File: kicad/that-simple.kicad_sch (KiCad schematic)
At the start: 20 parts

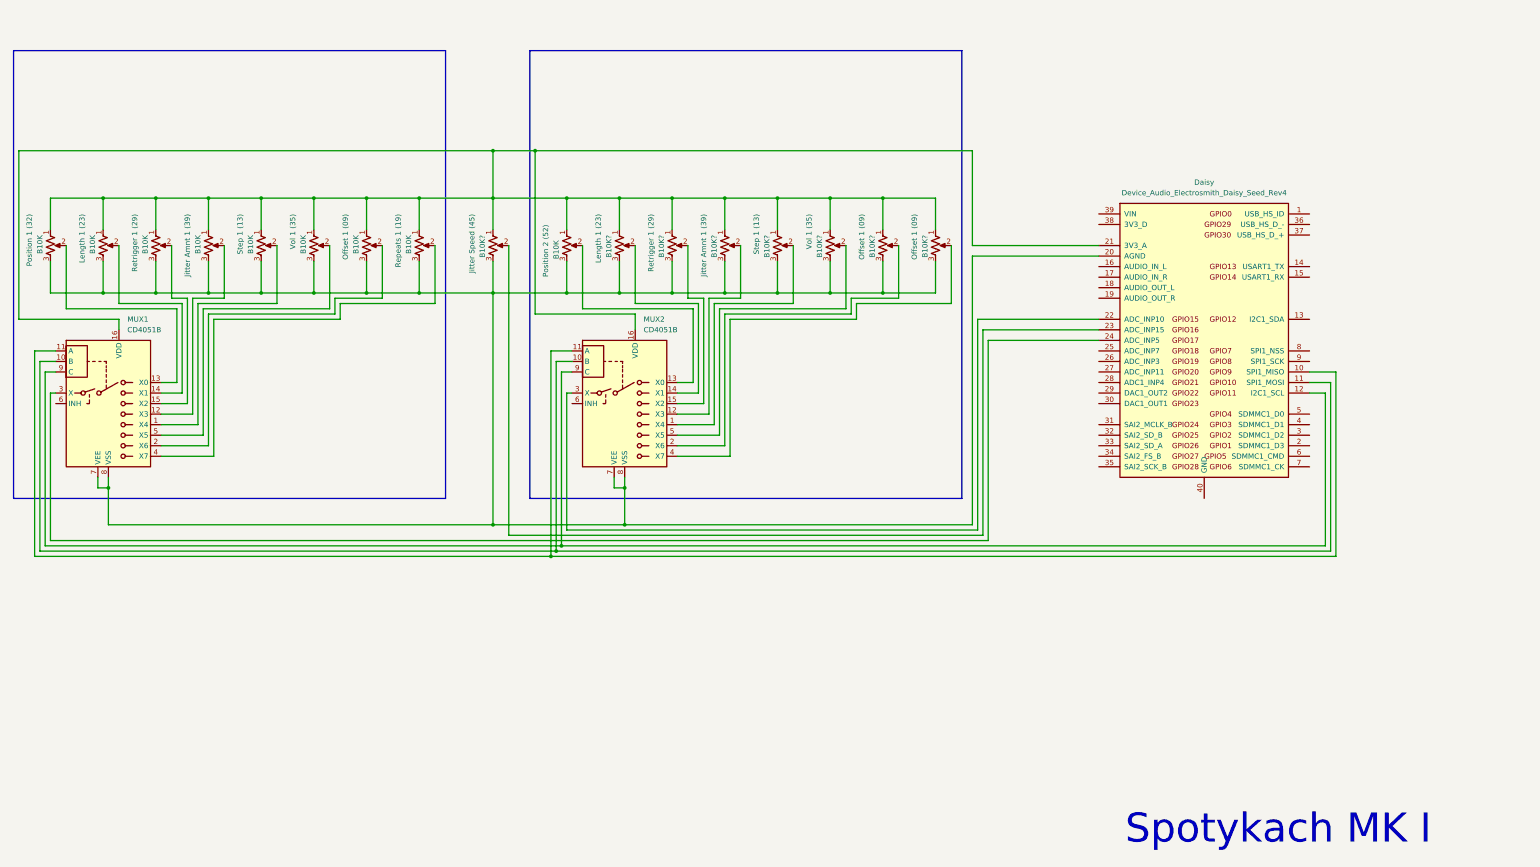
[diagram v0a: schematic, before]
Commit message: More complex
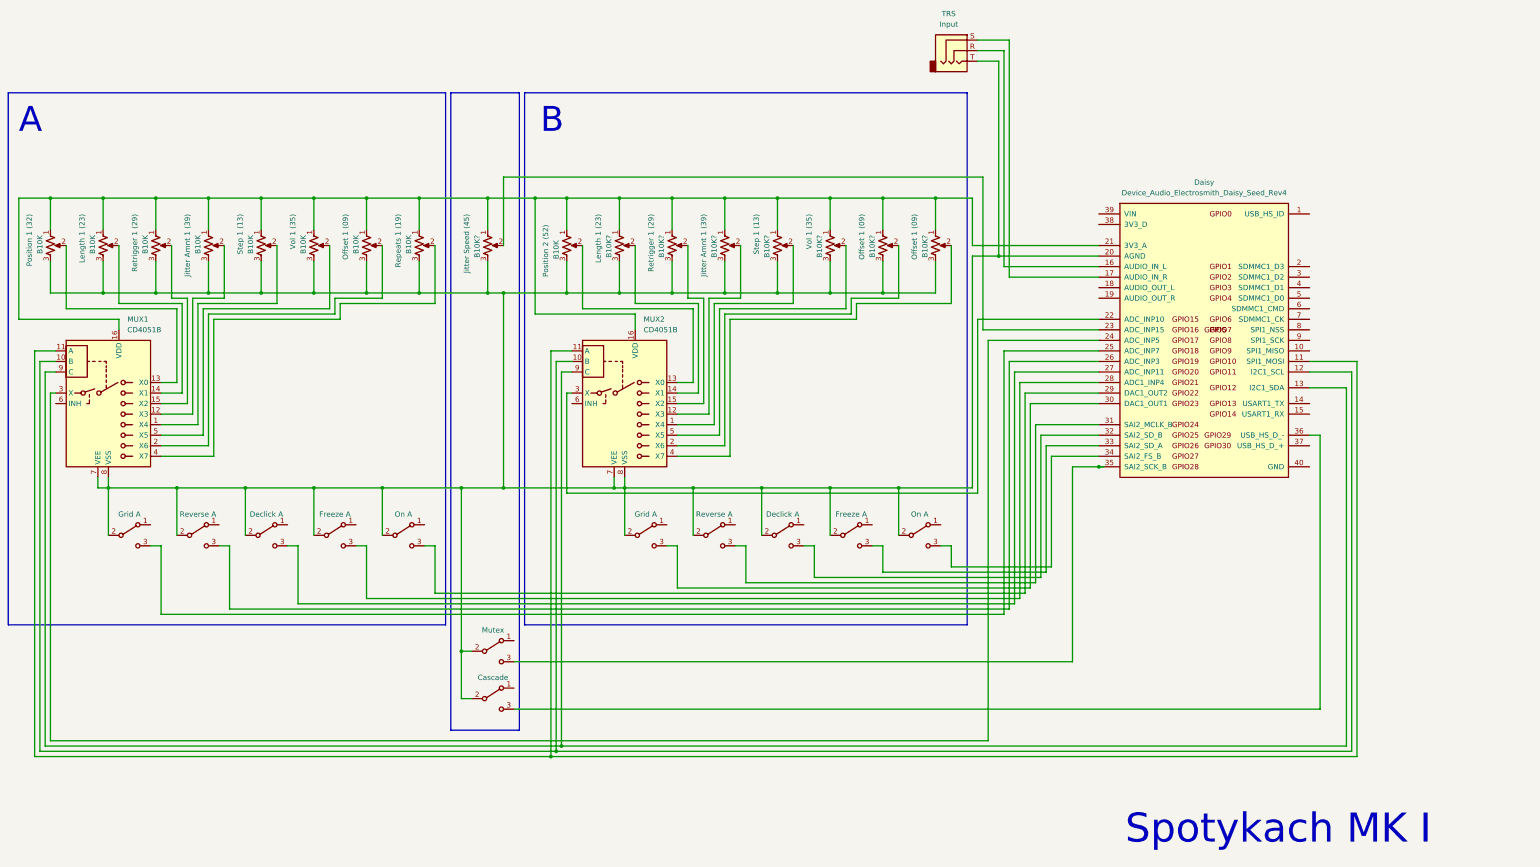
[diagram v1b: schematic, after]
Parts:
- added SPDT, SPDT?: Grid A, symbol Switch:SW_SPDT
- added SPDT?: Mutex, symbol Switch:SW_SPDT
- added SPDT? (x2): Declick A, symbol Switch:SW_SPDT
- added SPDT? (x2): Freeze A, symbol Switch:SW_SPDT
- added SPDT? (x2): On A, symbol Switch:SW_SPDT
- added SPDT?: Cascade, symbol Switch:SW_SPDT
- added SPDT? (x2): Reverse A, symbol Switch:SW_SPDT
- added TRS: Input, symbol Connector:AudioJack3
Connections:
- net at MUX1.10 (B), MUX2.10 (B): now also Daisy.12 (I2C1_SCL); no longer Daisy.11 (SPI1_MOSI)
- net at MUX1.11 (A), MUX2.11 (A): now also Daisy.11 (SPI1_MOSI); no longer Daisy.10 (SPI1_MISO)
- net at B10K.3, B10K.3, B10K.3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: now also SPDT.2 (B), SPDT?.2 (B), SPDT?.2 (B), SPDT?.2 (B), SPDT?.2 (B), SPDT?.2 (B), SPDT?.2 (B), SPDT?.2 (B), SPDT?.2 (B), SPDT?.2 (B), SPDT?.2 (B), SPDT?.2 (B), TRS.T
- net at MUX1.9 (C), MUX2.9 (C): now also Daisy.13 (I2C1_SDA); no longer Daisy.12 (I2C1_SCL)
- net at Daisy.16 (AUDIO_IN_L): now also TRS.R
- net at Daisy.17 (AUDIO_IN_R): now also TRS.S
- net at Daisy.25 (ADC_INP7): now also SPDT.3 (C)
- net at Daisy.26 (ADC_INP3): now also SPDT?.3 (C)
- net at Daisy.27 (ADC_INP11): now also SPDT?.3 (C)
- net at Daisy.28 (ADC1_INP4): now also SPDT?.3 (C)
- net at Daisy.29 (DAC1_OUT2): now also SPDT?.3 (C)
- net at Daisy.30 (DAC1_OUT1): now also SPDT?.3 (C)
- net at Daisy.31 (SAI2_MCLK_B): now also SPDT?.3 (C)
- net at Daisy.32 (SAI2_SD_B): now also SPDT?.3 (C)
- net at Daisy.33 (SAI2_SD_A): now also SPDT?.3 (C)
- net at Daisy.34 (SAI2_FS_B): now also SPDT?.3 (C)
- net at Daisy.35 (SAI2_SCK_B): now also SPDT?.3 (C)
- net at Daisy.36 (USB_HS_D_-): now also SPDT?.3 (C)
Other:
- note added: "A"
- note added: "B"
- moved on the sheet: B10K?, Daisy
